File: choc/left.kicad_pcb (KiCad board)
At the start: 2 copper layers, 117 x 92 mm, 63 parts, among them J1 USB_B_Micro, SW1 SW_Push, SW10 SW_Push, SW11 SW_Push, SW12 SW_Push, SW13 SW_Push, SW14 SW_Push, SW15 SW_Push, SW16 SW_Push, SW17 SW_Push, SW18 SW_Push, SW19 SW_Push, SW2 SW_Push, SW20 SW_Push, SW21 SW_Push, SW22 SW_Push, SW23 SW_Push, SW3 SW_Push, SW4 SW_Push, SW47 SW_Push, SW49 SW_Push, SW5 SW_Push, SW6 SW_Push, SW7 SW_Push, SW8 SW_Push, SW9 SW_Push, U1 ProMicro

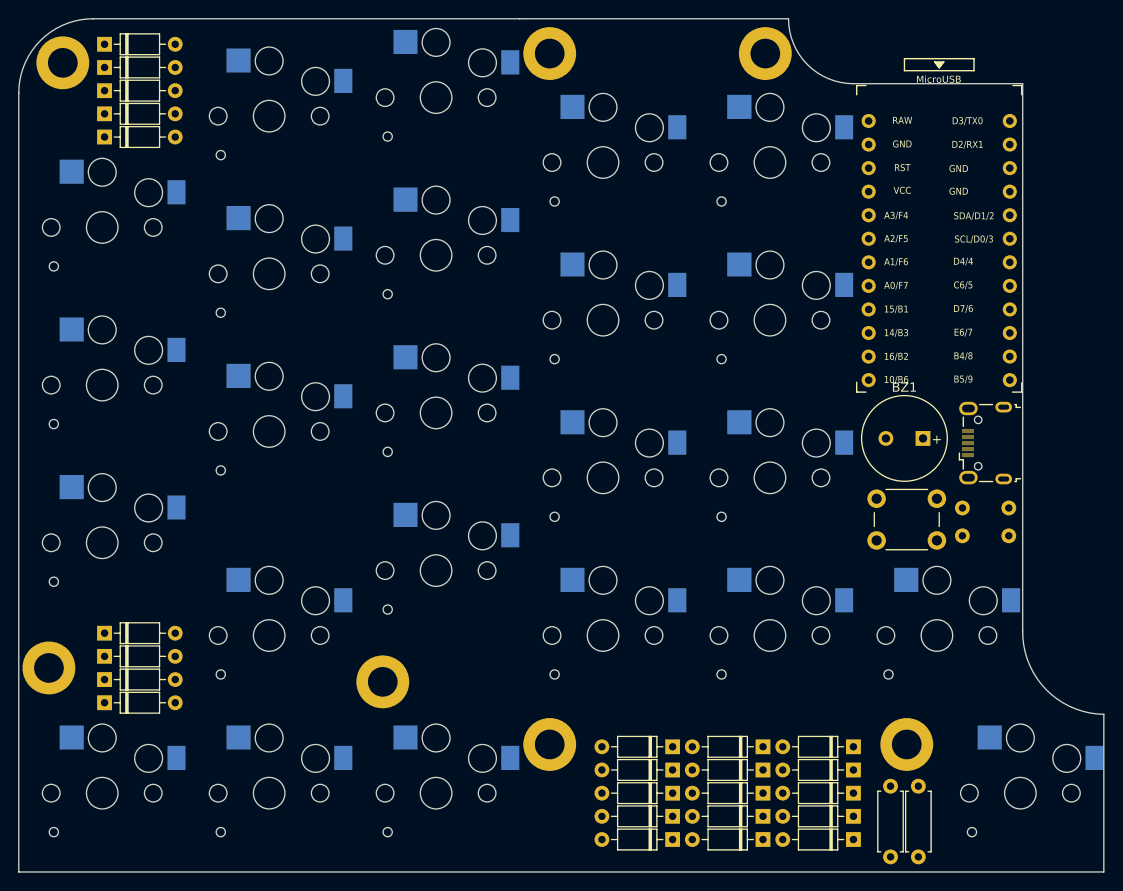
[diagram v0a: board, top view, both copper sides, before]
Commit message: import left ses
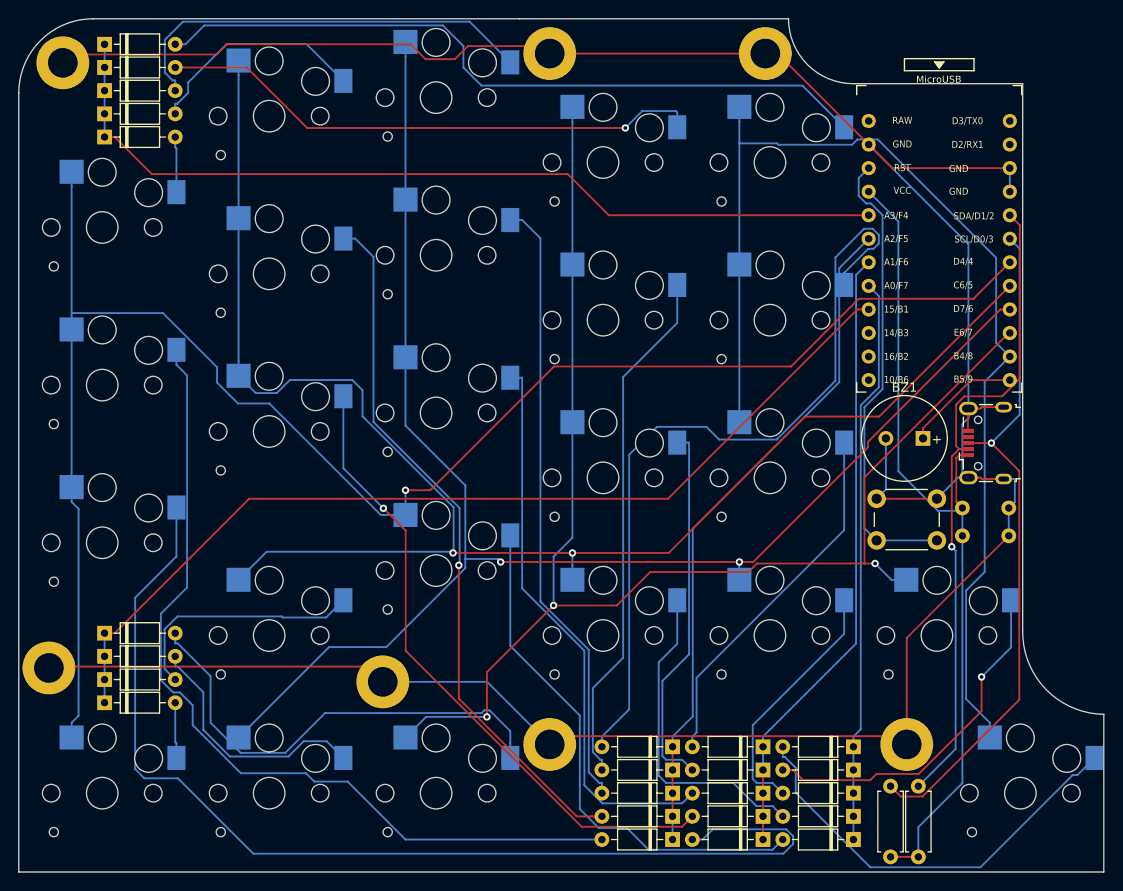
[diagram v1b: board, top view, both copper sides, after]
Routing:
- net GND: track 0.00 -> 311.9 mm
- net /lcol0: track 0.00 -> 185.6 mm, vias 0 -> 1
- net /lcol1: track 0.00 -> 170.1 mm, vias 0 -> 2
- net /lcol2: track 0.00 -> 163.8 mm, vias 0 -> 2
- net /lcol3: track 0.00 -> 151.3 mm, vias 0 -> 3
- net /lcol4: track 0.00 -> 122.6 mm
- net Net-(D3-Pad2): track 0.00 -> 117.7 mm
- net /lrow4: track 0.00 -> 104.4 mm
- net /lrow0: track 0.00 -> 95.9 mm
- net Net-(D2-Pad2): track 0.00 -> 93.2 mm
- net +5V: track 0.00 -> 89.8 mm
- net Net-(D21-Pad2): track 0.00 -> 86.2 mm
- net Net-(D20-Pad2): track 0.00 -> 78.9 mm
- net Net-(D7-Pad2): track 0.00 -> 76.3 mm, vias 0 -> 1
- net /lSCL: track 0.00 -> 73.8 mm, vias 0 -> 1
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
